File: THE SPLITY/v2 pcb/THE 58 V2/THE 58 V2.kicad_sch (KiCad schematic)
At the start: 136 parts, among them J1 Conn_01x02_Socket, J2 Conn_01x02_Socket, U1 Nice_Nano_V2, U2 Nice_Nano_V2, U3 TRRS, U4 TRRS

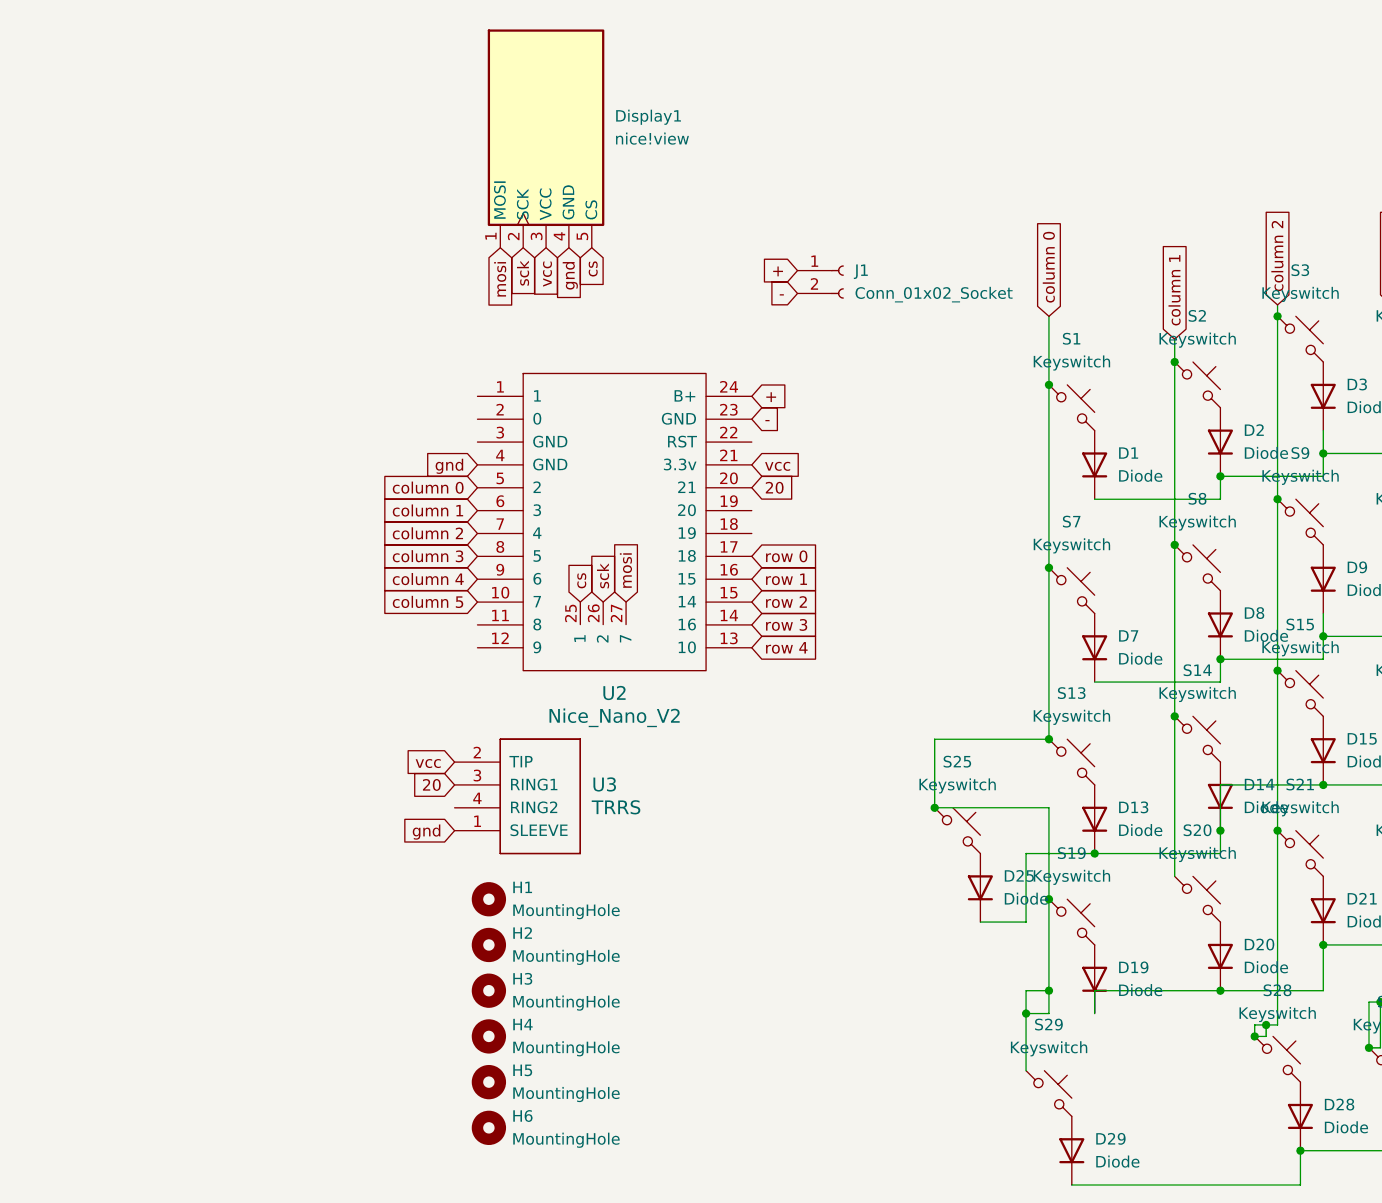
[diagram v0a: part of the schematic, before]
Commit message: v2
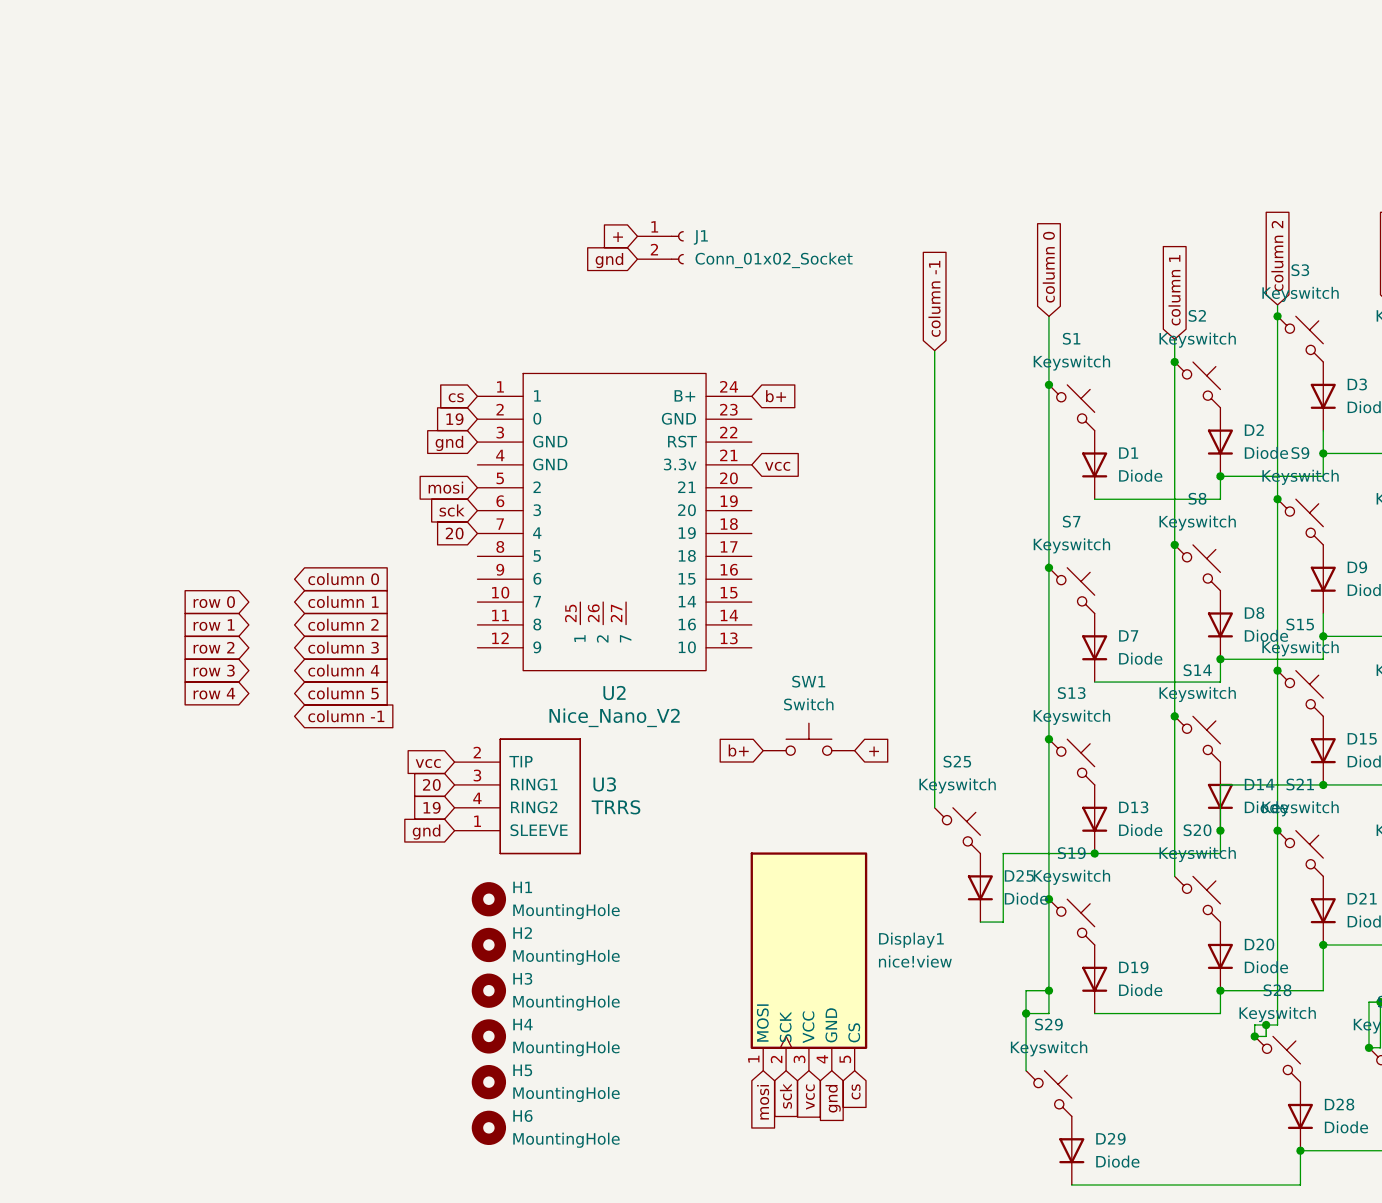
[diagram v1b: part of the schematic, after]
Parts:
- added SW1: Switch, ScottoKeebs_Components:Switch_MSK12C02, symbol ScottoKeebs:Placeholder_Switch
- Display1, Display2: footprint nice_view:nice_view -> nice view:nice_view
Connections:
- net +: now also SW1.2; no longer U2.24 (B+)
- net 20: now also U2.7 (4); no longer U2.20 (21)
- net column 0: no longer S25.1, U2.5 (2)
- net column 1: no longer U2.6 (3)
- net column 2: no longer U2.7 (4)
- net column 3: no longer U2.8 (5)
- net column 4: no longer U2.9 (6)
- net column 5: no longer U2.10 (7)
- net cs: now also U2.1; no longer U2.25 (1)
- net gnd: now also J1.2 (Pin_2), U2.3 (GND); no longer U2.4 (GND)
- net mosi: now also U2.5 (2); no longer U2.27 (7)
- net row 0: no longer U2.17 (18)
- net row 1: no longer U2.16 (15)
- net row 2: no longer U2.15 (14)
- net row 3: no longer U2.14 (16)
- net row 4: no longer U2.13 (10)
- net sck: now also U2.6 (3); no longer U2.26 (2)
- net 19: now reaches U3.4 (RING2)
- net 19: now also U2.2 (0)
- net -: no longer names the net of U2.23 (GND)
- net -: no longer J1.2 (Pin_2)
- new net b+: SW1.1, U2.24 (B+)
- new net column -1: S25.1
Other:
- moved on the sheet: Display1, J1
